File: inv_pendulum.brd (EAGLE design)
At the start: 49.2 x 74.9 mm, 9 parts

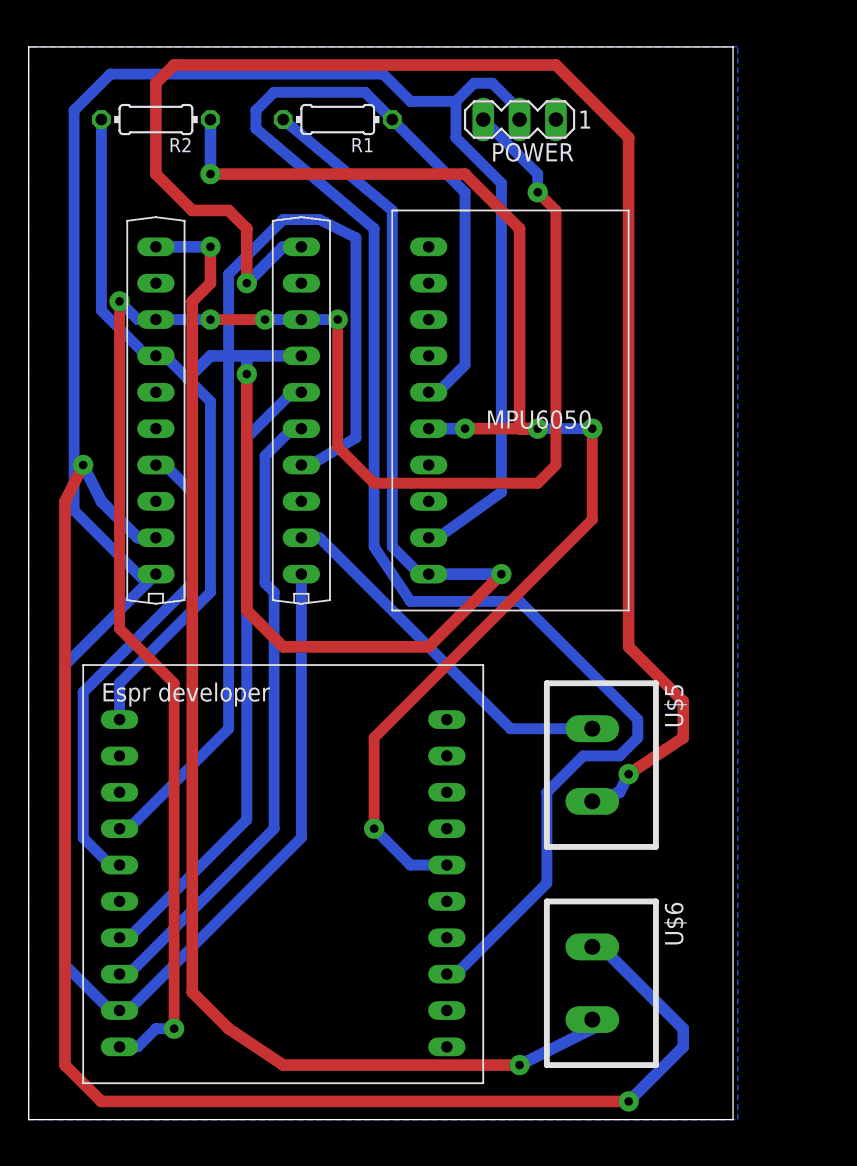
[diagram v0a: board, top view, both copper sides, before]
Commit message: update design
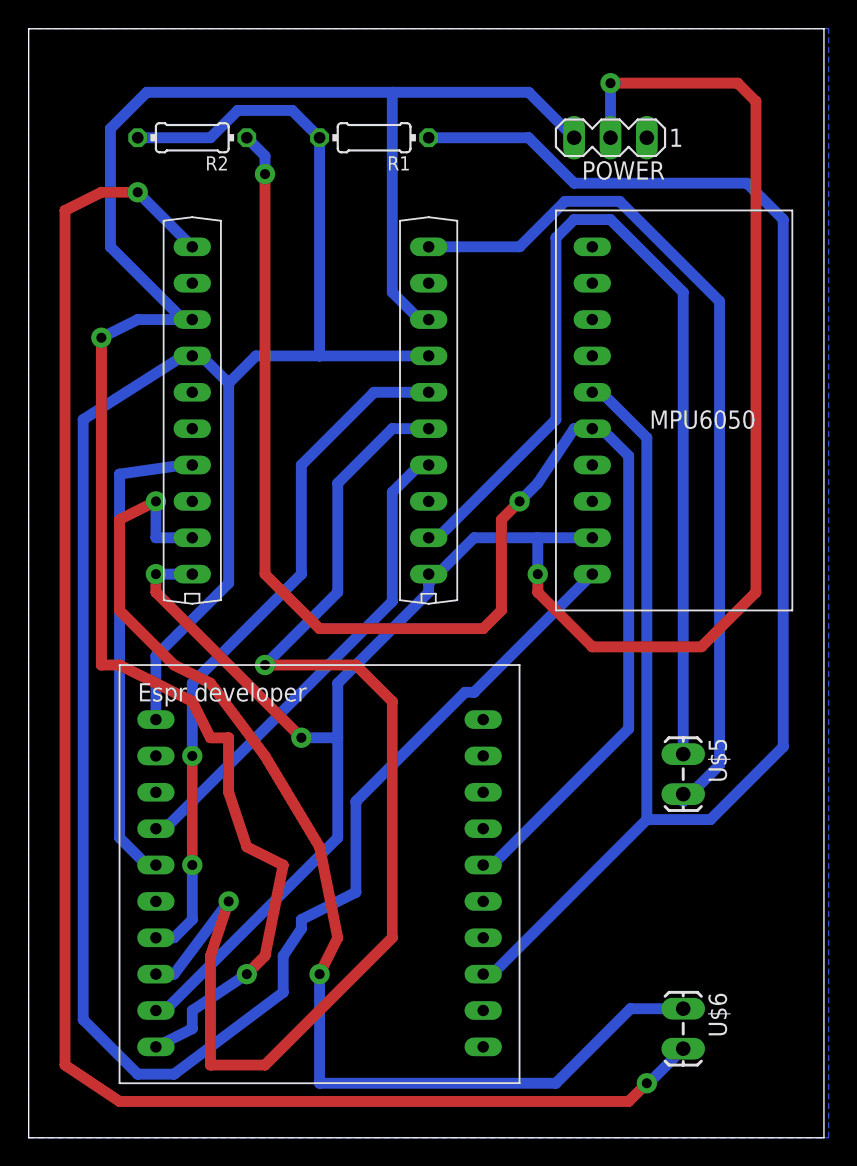
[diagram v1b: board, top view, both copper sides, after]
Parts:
- U$5, U$6: value TBLOCK-2 -> (none); device akizuki_MOSFET:TBLOCK-2 -> SparkFun-Connectors:1X02_LOCK_LONGPADS
- moved U$1 11.4 mm to (44.5, 49.5)
- moved U$3 8.89 mm to (27.9, 49.5)
- moved U$5 6.48 mm to (45.7, 25.4)
- moved U$6 6.48 mm to (45.7, 7.62)
- moved POWER 6.48 mm to (40.6, 68.6)
- moved R1 2.84 mm to (24.1, 68.6)
- moved R2 2.84 mm to (11.4, 68.6)
- moved U$2 2.54 mm to (24.1, 16.5)
- moved U$4 2.54 mm to (11.4, 49.5)
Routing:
- net N$5: track 110.1 -> 61.0 mm, vias 2 -> 0
- net 3V3: track 137.6 -> 180.6 mm, vias 2 -> 0
- net N$4: track 25.8 -> 68.8 mm
- net IN1: track 44.6 -> 84.8 mm, vias 0 -> 2
- net PWM1: track 71.3 -> 34.0 mm
- net GND: track 175.9 -> 143.2 mm, vias 0 -> 4
- net N$11: track 87.4 -> 115.9 mm
- net N$10: track 105.7 -> 80.7 mm
- net 6V: track 124.4 -> 136.3 mm, vias 6 -> 2
- net SCL: track 94.0 -> 101.9 mm, vias 5 -> 2
- net SDA: track 116.8 -> 123.3 mm
- net IN2: track 44.1 -> 49.0 mm, vias 0 -> 2
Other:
- board size 49.2 x 74.9 mm -> 55.5 x 77.5 mm
